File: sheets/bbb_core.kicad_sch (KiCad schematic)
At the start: 11 parts, among them P10 BeagleBone_Black_Header, P11 BeagleBone_Black_Header, SW2 SW_DIP_x02, U2 CAT24C256

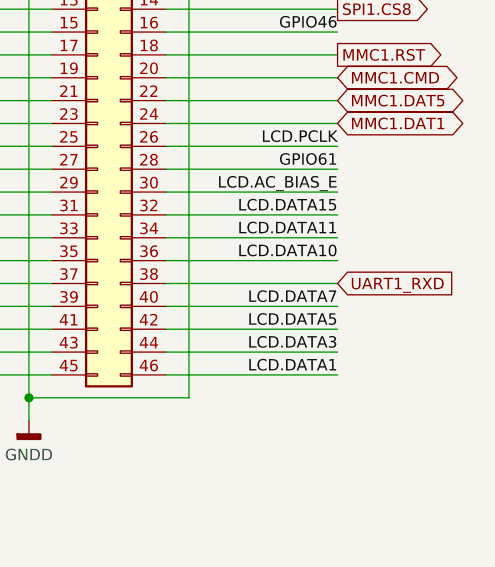
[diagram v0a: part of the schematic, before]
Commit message: Update bbb_core.kicad_sch
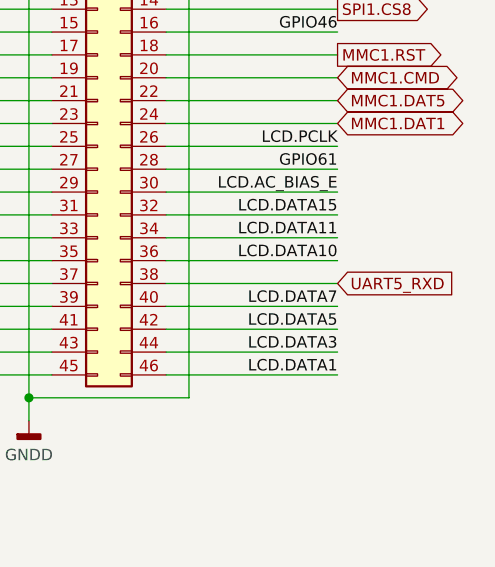
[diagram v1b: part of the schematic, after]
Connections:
- net UART1_RXD: no longer P11.38 (Pin_38)
- new net UART5_RXD: P11.38 (Pin_38)
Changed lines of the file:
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@@
 		)
 	)
-	(global_label "UART1_RXD"
+	(global_label "UART5_RXD"
 		(shape input)
 		(at 238.76 78.74 0)
